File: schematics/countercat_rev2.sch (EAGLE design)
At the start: 48 parts, among them Q1 2N3904, Q2 IRF520, Q3 IRF520, Q4 IRF520, U2 74HC04_HEX_INVERTER, U3 USD-SOCKETNEW, U4 ATMEGA328P_PDIP, Y1 16MHz

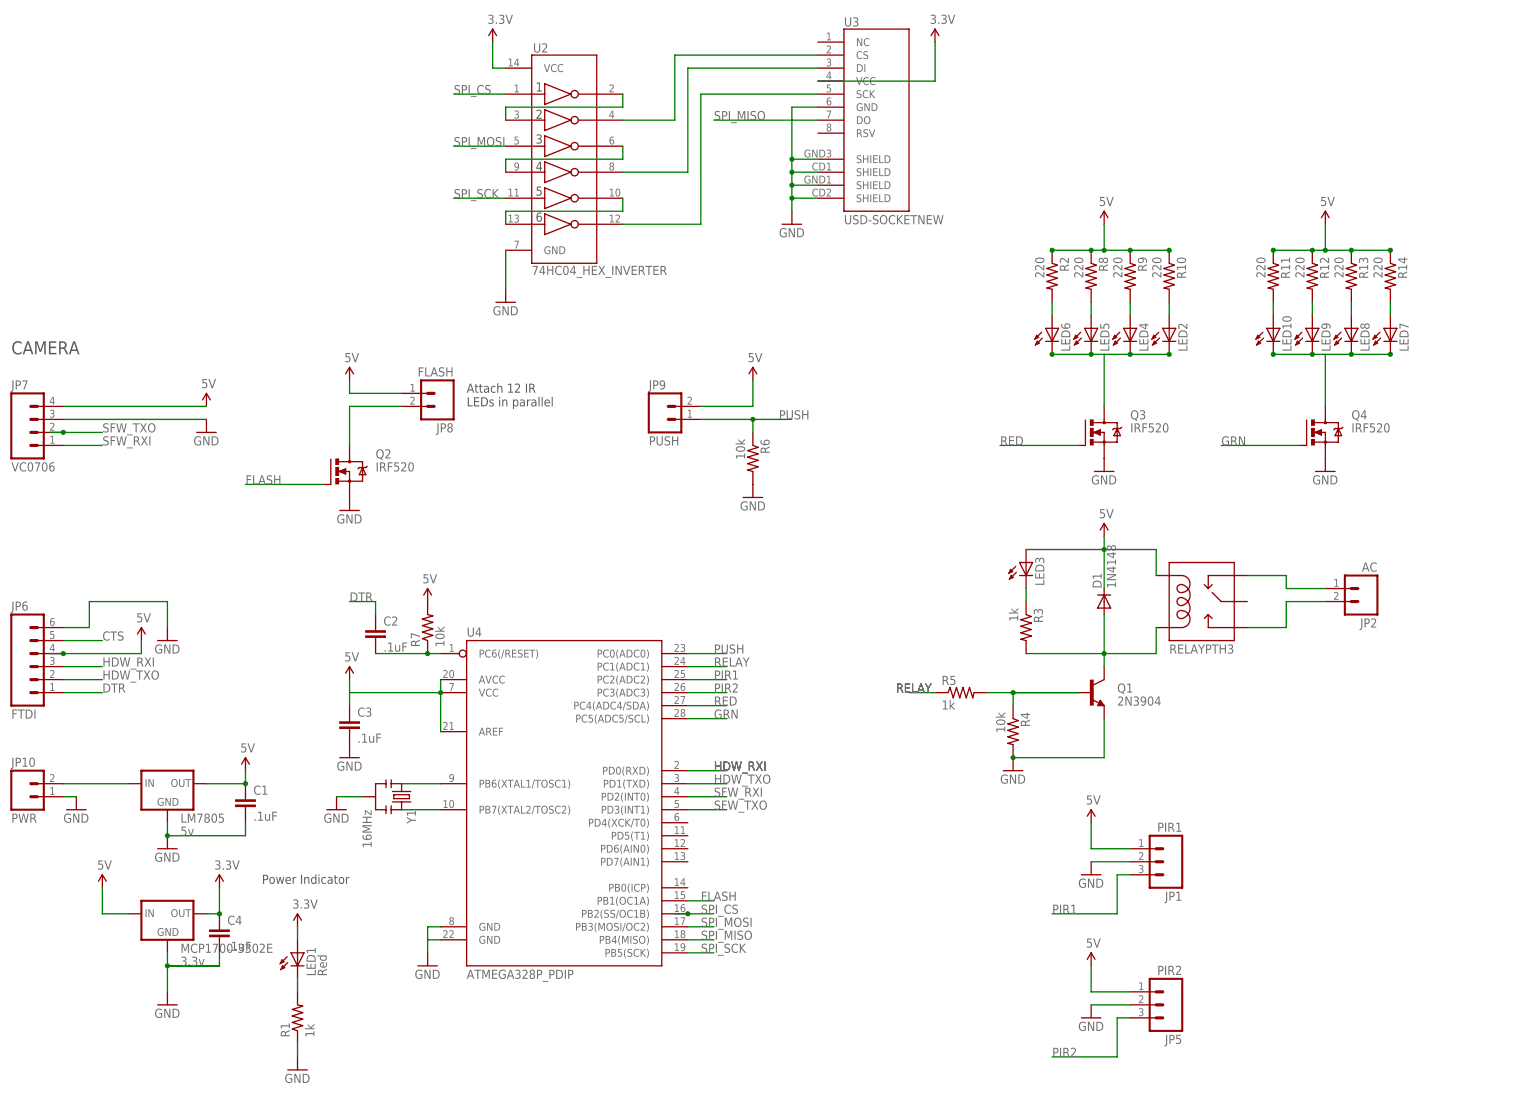
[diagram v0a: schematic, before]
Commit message: Started board design
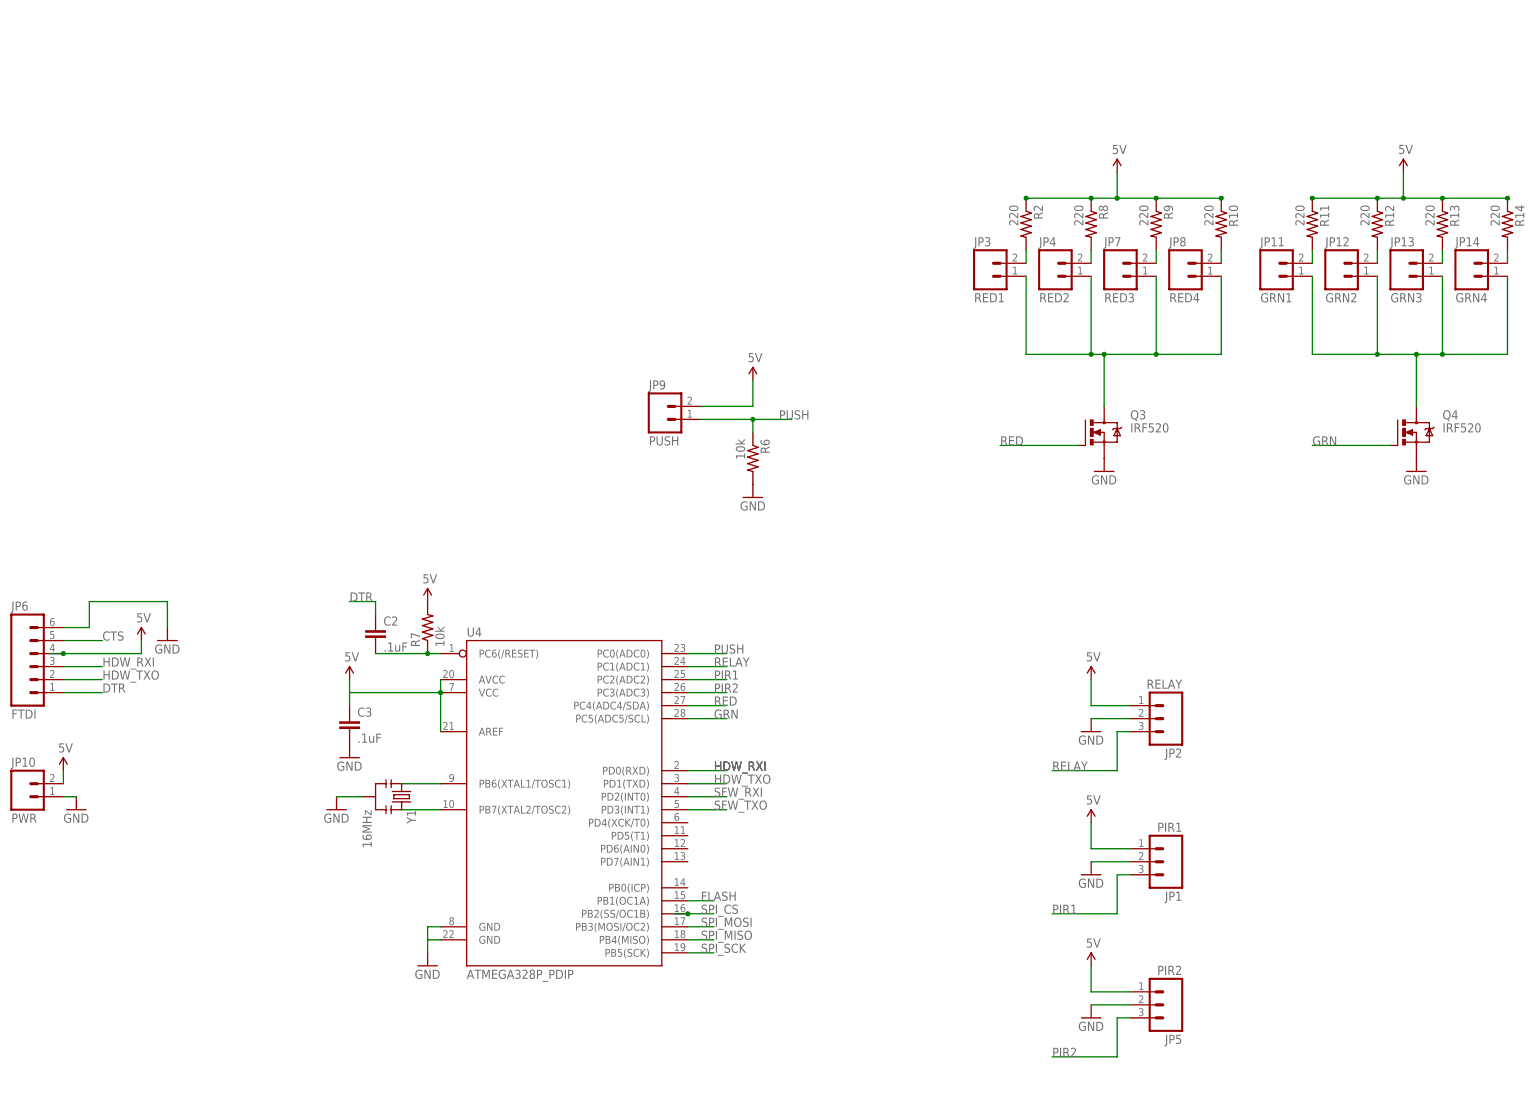
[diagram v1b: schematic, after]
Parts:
- removed C1, C4: .1uF, SparkFun-Capacitors:CAPPTH2
- removed D1: 1N4148, SparkFun:DIODEPTH
- removed LED1: Red, SparkFun-LED:LED3MM
- removed LED10, LED2, LED3, LED4, LED5, LED6, LED7, LED8, LED9: (no value), nick_DC2011:LED3MM
- removed LM7805: 5v, SparkFun-PowerIC:V_REG_78XXSINK
- removed MCP1700-3302E: 3.3v, SparkFun-PowerIC:V_REG_78XXTO-92_UNTESTED
- removed Q1: 2N3904, SparkFun:TRANSISTOR_NPNTO92
- removed Q2: IRF520, transistor-power:IRF520
- removed R1, R3, R5: 1k, SparkFun-Resistors:RESISTORPTH-1/4W
- removed R4: 10k, SparkFun-Resistors:RESISTORPTH-1/4W
- removed U$2: RELAYPTH3, SparkFun:RELAYPTH3
- removed U2: 74HC04_HEX_INVERTER, SparkFun-DigitalIC:74HC04_HEX_INVERTER
- removed U3: USD-SOCKETNEW, SparkFun:USD-SOCKETNEW
- added JP11: GRN1, SparkFun:M02POLAR
- added JP12: GRN2, SparkFun:M02POLAR
- added JP13: GRN3, SparkFun:M02POLAR
- added JP14: GRN4, SparkFun:M02POLAR
- added JP3: RED1, SparkFun:M02POLAR
- added JP4: RED2, SparkFun:M02POLAR
- JP2: value AC -> RELAY; device NickDC2011Breakouts:M025MM -> SparkFun:M03POLAR
- JP7: value VC0706 -> RED3; device SparkFun-Connectors:M04POLAR -> SparkFun:M02POLAR
- JP8: value FLASH -> RED4
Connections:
- removed net 3.3V: C4.1, LED1.A, MCP1700-3302E.OUT, U2.VCC, U3.VCC
- removed net N$1: LED3.C, R3.1
- removed net N$10: D1.A, Q1.C, R3.2, U$2.COIL2
- removed net N$11: Q1.B, R4.1, R5.2
- removed net N$14: LED1.C, R1.2
- removed net N$17: U2.5Y, U2.6A
- removed net N$20: U2.2Y, U3.CS
- removed net N$23: LED10.C, LED7.C, LED8.C, LED9.C, Q4.D
- removed net N$24: LED10.A, R11.2
- removed net N$25: LED9.A, R12.2
- removed net N$26: LED8.A, R13.2
- removed net N$27: LED7.A, R14.2
- removed net N$6: JP2.1, U$2.NC
- removed net N$9: JP2.2, U$2.NO
- removed net VB: JP10.2, LM7805.IN
- net 5V: now also JP10.2, JP2.1; no longer C1.1, D1.C, JP7.4, JP8.1, LED3.A, LM7805.OUT, MCP1700-3302E.IN, U$2.COIL1
- net FLASH: no longer Q2.G
- net GND: now also JP2.2; no longer C1.2, C4.2, JP7.3, LM7805.GND, MCP1700-3302E.GND, Q1.E, Q2.S, R1.1, R4.2, U2.GND, U3.GND, U3.SHIELD@1, U3.SHIELD@2, U3.SHIELD@3, U3.SHIELD@4
- net N$13: now also JP12.2, R12.2; no longer U2.4Y, U3.DI
- net N$15: now also JP13.2, R13.2; no longer U2.6Y, U3.SCK
- net N$16: now also JP14.2, R14.2; no longer U2.3Y, U2.4A
- net N$18: now also JP3.2; no longer LED6.A
- net N$19: now also JP4.2; no longer LED5.A
- net N$2: now also JP3.1, JP4.1, JP7.1, JP8.1; no longer LED2.C, LED4.C, LED5.C, LED6.C
- net N$21: now also JP7.2; no longer LED4.A
- net N$22: now also JP8.2; no longer LED2.A
- net N$4: now also JP11.1, JP12.1, JP13.1, JP14.1; no longer JP8.2, Q2.D
- net N$5: now also JP11.2, R11.2; no longer U2.1Y, U2.2A
- net RELAY: now also JP2.3; no longer R5.1
- net SFW_RXI: no longer JP7.1
- net SFW_TXO: no longer JP7.2
- net SPI_CS: no longer U2.1A
- net SPI_MISO: no longer U3.DO
- net SPI_MOSI: no longer U2.3A
- net SPI_SCK: no longer U2.5A
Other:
- note removed: "Attach 12 IR LEDs in parallel"
- note removed: "CAMERA"
- note removed: "Power Indicator"
- moved on the sheet: JP8, Q4, R10, R11, R12, R13, R14, R2, R8, R9
